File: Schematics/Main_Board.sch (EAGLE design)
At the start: 30 parts, among them IC1 LM317MBSTT3, IC2 LM317MBSTT3, X1 MINI-USB-32005-201, X2 RJ45-6L-B

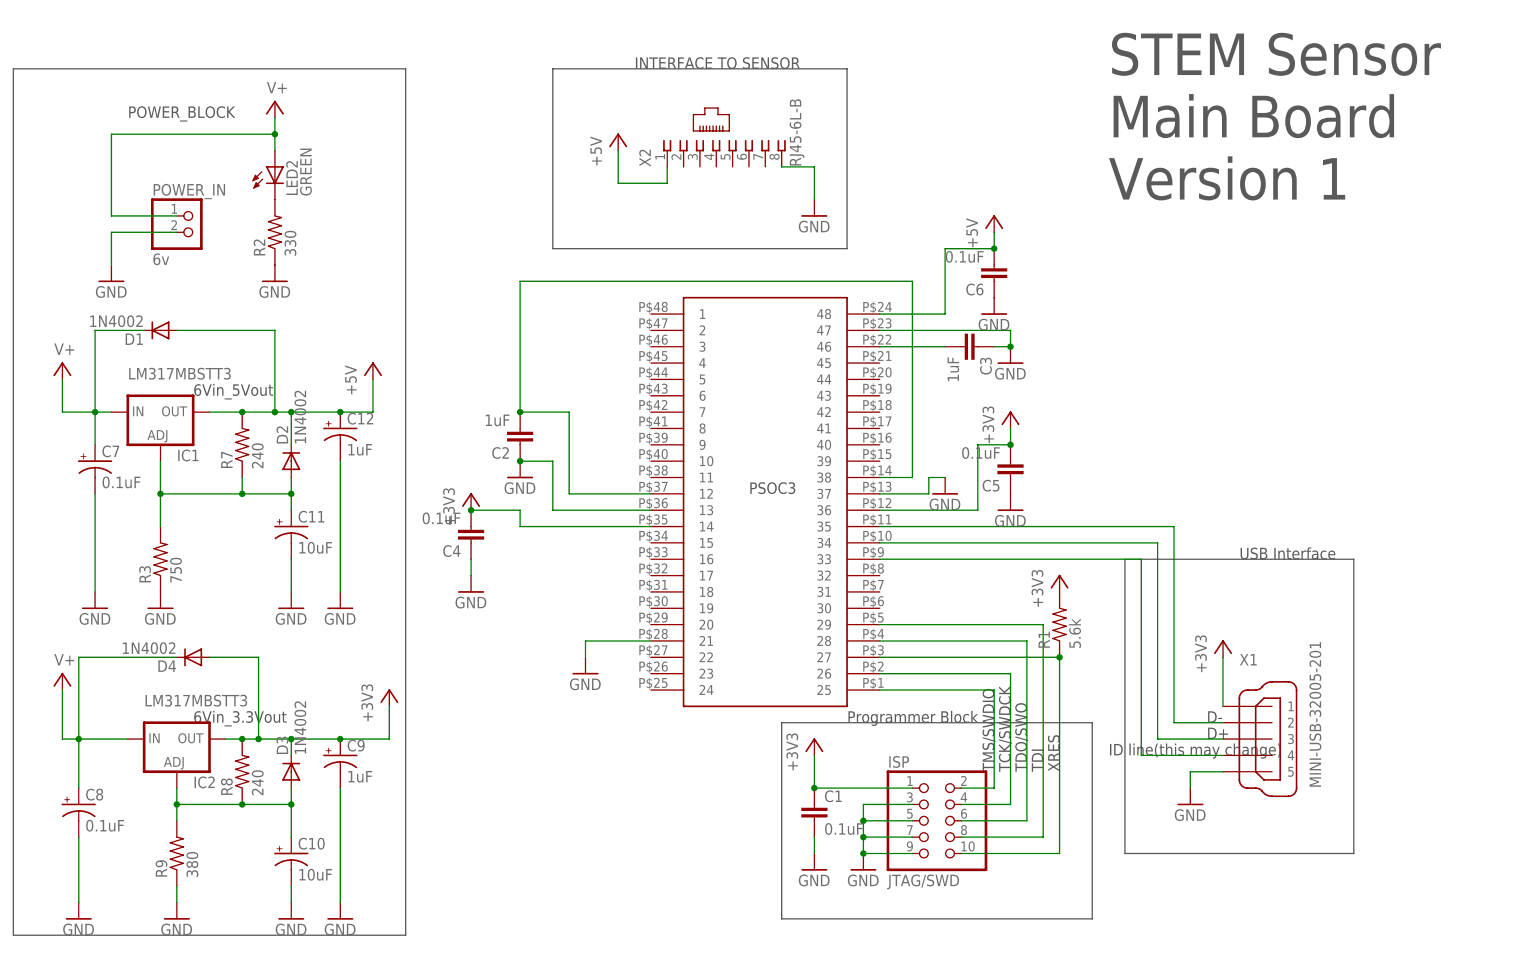
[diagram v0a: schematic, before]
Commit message: Updated Schematic
Grounds and voltages are not set yet.  Most are place holders for the
moment.
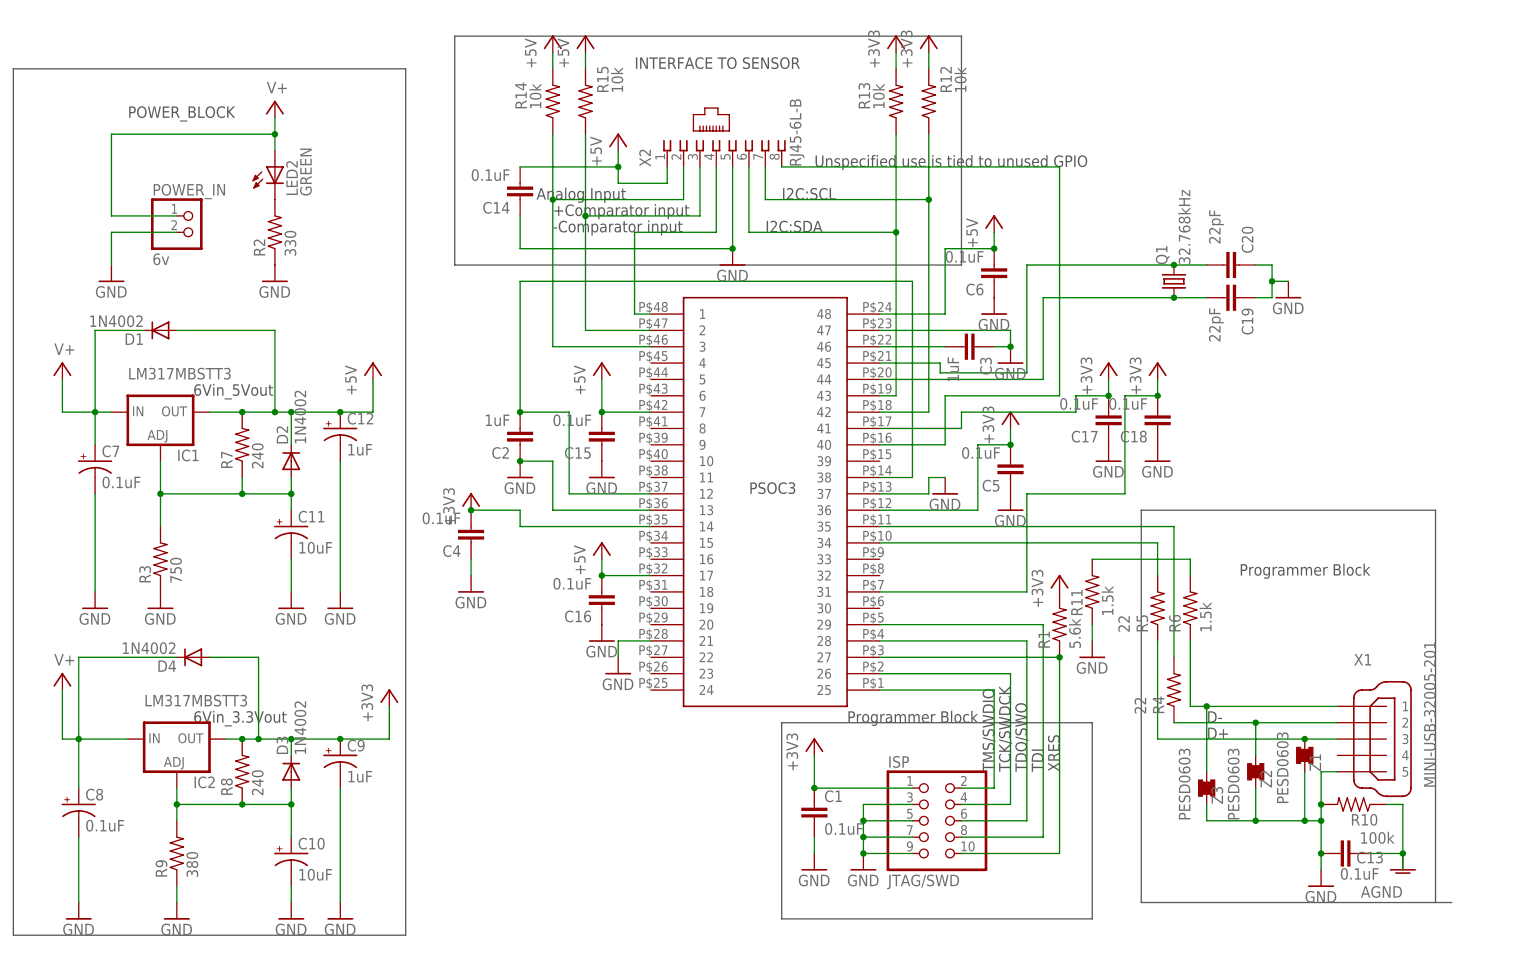
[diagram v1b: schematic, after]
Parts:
- added C13, C14, C15, C16, C17, C18: 0.1uF, rcl:C-EUC1206
- added C19, C20: 22pF, rcl:C-EUC1206
- added Q1: 32.768kHz, crystal:CRYSTALHC18U-V
- added R10: 100k, rcl:R-US_M1206
- added R11, R6: 1.5k, rcl:R-US_M1206
- added R12, R13, R14, R15: 10k, rcl:R-US_R0603
- added R4, R5: 22, rcl:R-US_M1206
- added Z1, Z2, Z3: PESD0603, supressor:PESD0603
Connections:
- new net AGND: C13.1, R10.1
- new net ANALOGINPUT: R14.1, U$1.3, X2.2
- new net N$13: R5.1, X1.3, Z1.2
- new net N$14: R4.1, X1.2, Z2.2
- new net N$16: C20.2, Q1.2, U$1.45
- new net N$17: R6.1, X1.1, Z3.2
- new net N$18: R15.1, U$1.2, X2.3
- new net N$19: U$1.1, X2.4
- new net N$20: R13.1, U$1.43, X2.6
- new net N$21: R12.1, U$1.42, X2.7
- new net N$22: U$1.40, X2.8
- new net N$23: C19.2, Q1.1, U$1.44
- net +3V3: now also C17.2, C18.2, R12.2, R13.2, U$1.31, U$1.41; no longer X1.1
- net +5V: now also C14.2, C15.2, C16.2, R14.2, R15.2, U$1.17, U$1.7
- net GND: now also C13.2, C14.1, C15.1, C16.1, C17.1, C18.1, C19.1, C20.1, R10.2, R11.1, X2.5, Z1.1, Z2.1, Z3.1; no longer X2.8
- net N$1: now also R4.2; no longer X1.2
- net N$2: now also R5.2; no longer X1.3
- net N$3: now also R11.2, R6.2; no longer U$1.33, X1.4
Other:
- note added: "+Comparator input"
- note added: "-Comparator input"
- note added: "Analog Input"
- note added: "I2C:SCL"
- note added: "I2C:SDA"
- note added: "Unspecified use is tied to unused GPIO"
- note removed: "ID line(this may change)"
- note removed: "STEM Sensor Main Board Version 1"
- note removed: "USB Interface"
- moved on the sheet: X1
